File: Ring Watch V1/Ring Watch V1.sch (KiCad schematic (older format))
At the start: 12 parts, among them J1 Programming Header, J2 CR2023 Socket, U1 ATtiny85-20SU, U2 PCF8523T, Y1 32.768

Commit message: more layout changes
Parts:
- H1: footprint TestPoint:TestPoint_Pad_4.0x4.0mm -> TestPoint:TestPoint_Keystone_5019_Minature
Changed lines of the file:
@@
 F 0 "H1" V 2237 2153 50  0000 C CNN
 F 1 "Battery Mechanical Switch Pad" V 2146 2153 50  0000 C CNN
-F 2 "TestPoint:TestPoint_Pad_4.0x4.0mm" H 2000 2150 50  0001 C CNN
+F 2 "TestPoint:TestPoint_Keystone_5019_Minature" H 2000 2150 50  0001 C CNN
 F 3 "~" H 2000 2150 50  0001 C CNN
 	1    2000 2150

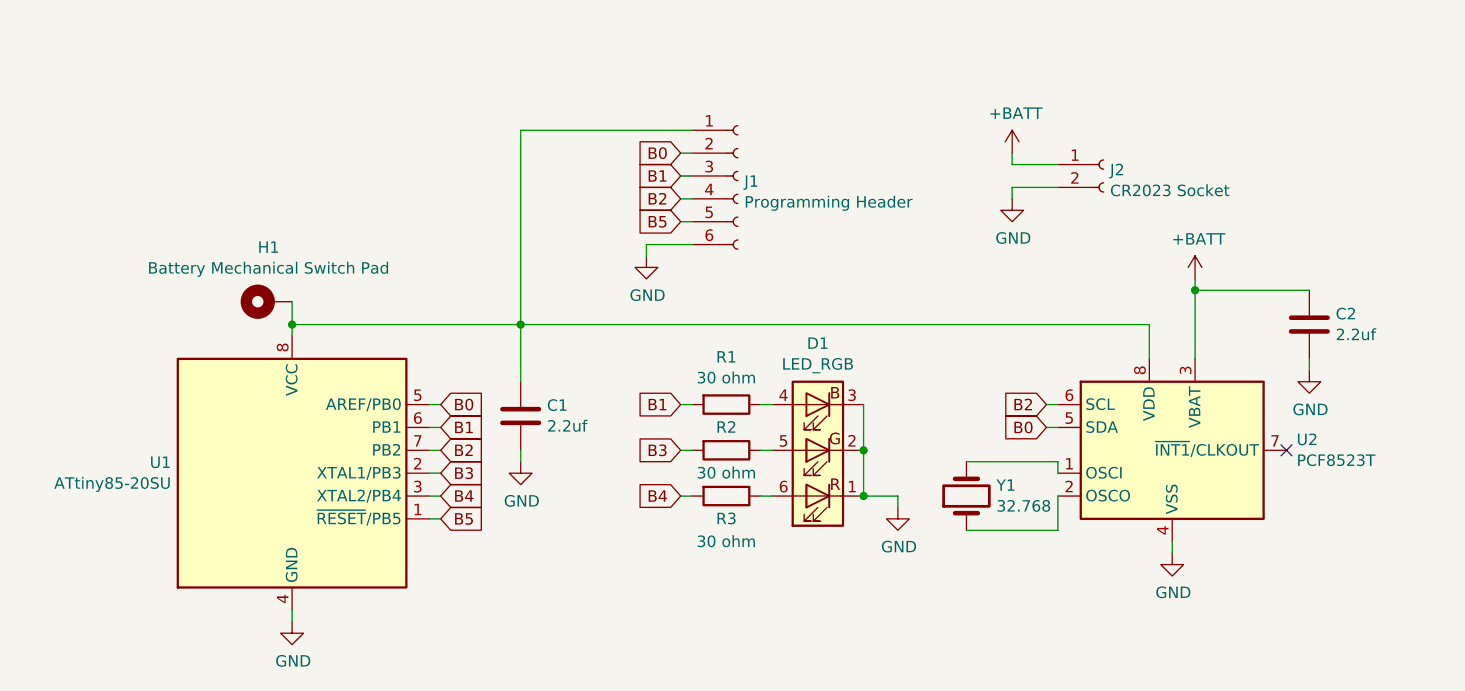
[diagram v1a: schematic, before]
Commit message: minor changes, need to place GND polygons
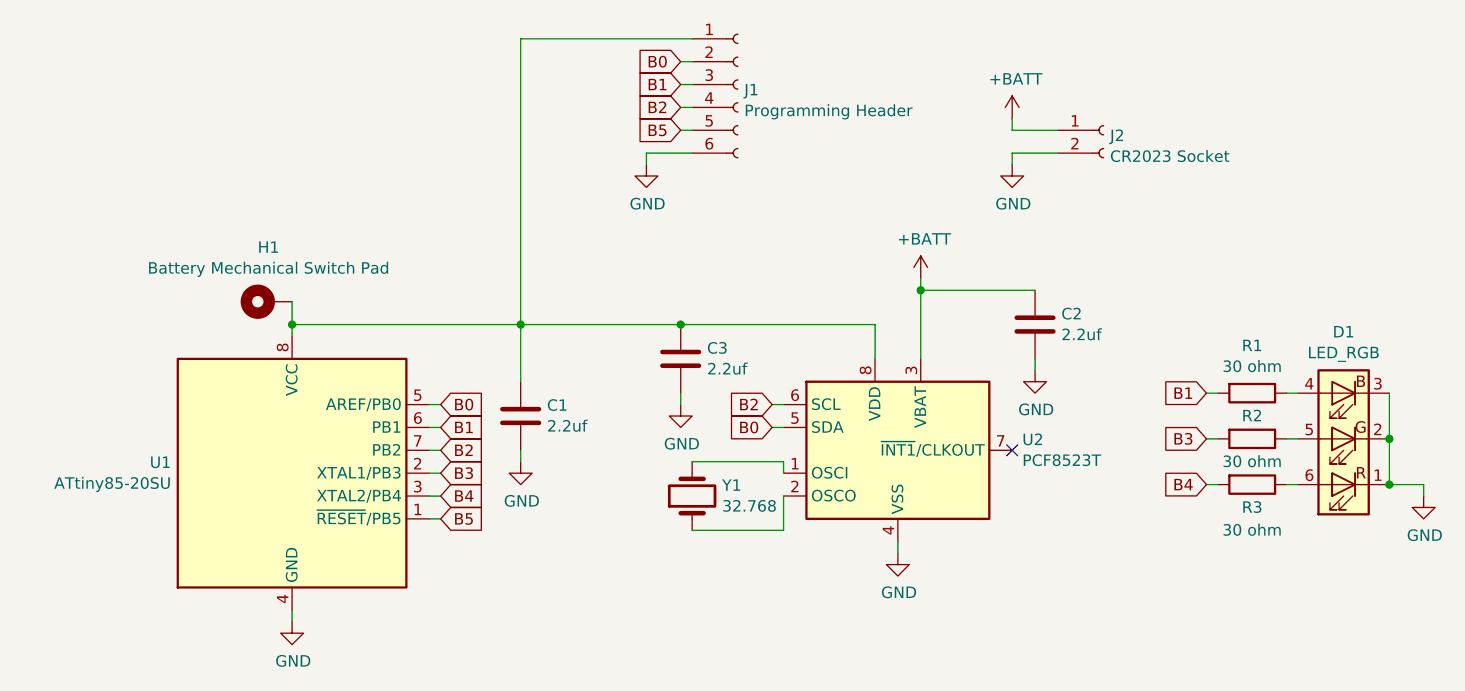
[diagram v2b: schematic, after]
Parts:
- added C3: 2.2uf, Capacitor_SMD:C_0805_2012Metric_Pad1.15x1.40mm_HandSolder, symbol Device:C
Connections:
- net GND: now also C3.2
- net at C1.1, H1.1, J1.1 (Pin_1)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: now also C3.1
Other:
- moved on the sheet: C2, D1, J1, J2, R1, R2, R3, U2, Y1
